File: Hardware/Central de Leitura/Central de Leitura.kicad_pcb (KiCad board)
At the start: 2 copper layers, 142.8 x 126.5 mm, 10 parts, among them J1 Bateria, J2 Fonte, J3 Modulo ZMPT101B, Q1 BC338, U1 Módulo TP4056, U2 E32-433T20D, U3 ESP32-C6-DevKitC-1

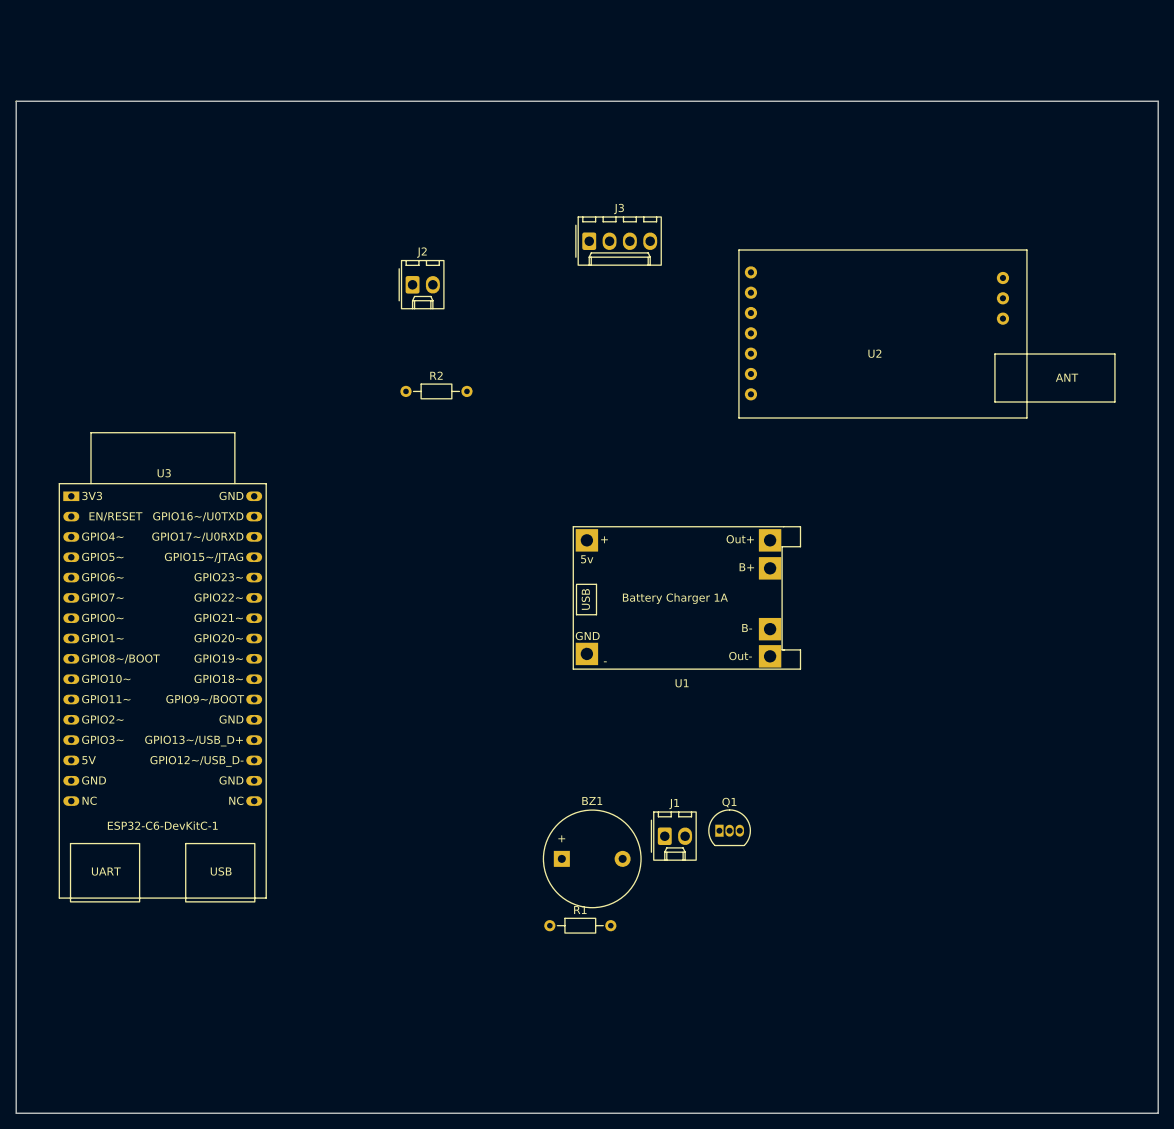
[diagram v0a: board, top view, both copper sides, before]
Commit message: Pequenos ajustes
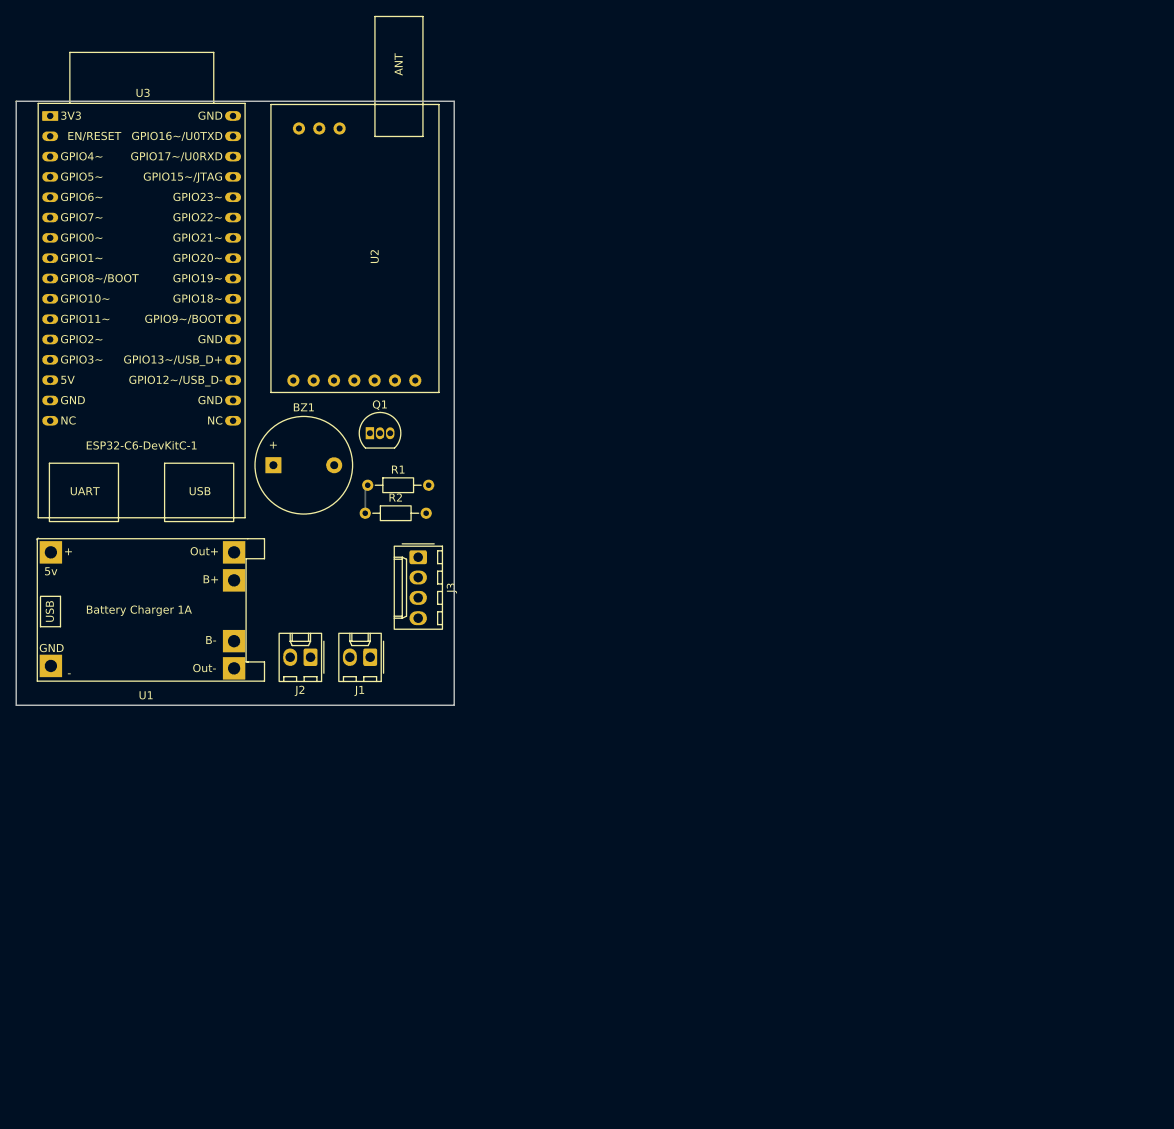
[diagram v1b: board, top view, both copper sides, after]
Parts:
- moved U1 67.0 mm to (43.9, 85.2)
- moved Q1 66.2 mm to (85.5, 72.0)
- moved U2 61.2 mm to (73.1, 66.9), turned to 90 degrees
- moved BZ1 61.0 mm to (73.4, 76.0)
- moved R1 59.6 mm to (85.2, 78.5)
- moved J2 48.3 mm to (78.0, 100.0), turned to 180 degrees
- moved U3 47.6 mm to (45.5, 32.3)
- moved J3 44.9 mm to (91.5, 87.5), turned to -90 degrees
- moved J1 43.1 mm to (85.5, 100.0), turned to 180 degrees
- moved R2 16.1 mm to (84.9, 82.0)
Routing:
- net Buzzer: track 0.00 -> 3.65 mm
- net GND: track 0.00 -> 1.36 mm
- net Net-(Q1-B): track 0.00 -> 0.67 mm
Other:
- board size 142.8 x 126.5 mm -> 54.8 x 75.5 mm
